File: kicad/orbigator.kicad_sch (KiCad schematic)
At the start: 0 parts

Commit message: KiCad schematic WiP
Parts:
- added BT1: CR2032, symbol Device:Battery_Cell
- added DISP1: OLED_Encoder, symbol orbigator:OLED_Encoder
- added M1: DYNAMIXEL_1, symbol Connector_Generic:Conn_01x03
- added M2: DYNAMIXEL_2, symbol Connector_Generic:Conn_01x03
- added R1, R2, R3: 10k, symbol PCM_Elektuur:R
- added RTC1: DS3232, symbol orbigator:Adafruit_DS3231_Breakout
- added U1: Pico_2, Module_RaspberryPi_Pico:RaspberryPi_Pico_Original_SMD_HandSolder, symbol MCU_Module_RaspberryPi_Pico:RaspberryPi_Pico_DebugPins
- added U2: 74LS126, symbol 74xx:74LS126
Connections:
- new net 3V3: DISP1.9 (VCC), R2.1 (+), R3.1 (+), RTC1.1 (Vin), U1.36 (3V3), U2.14 (VCC)
- new net 3V_BAT: BT1.1 (+), RTC1.5 (BAT)
- new net 5V0: M1.2 (Pin_2), M2.2 (Pin_2), R1.1 (+), U1.40 (VBUS)
- new net 5V_SYS: U1.39 (VSYS)
- new net BAK_BTN: DISP1.7 (BAK_BTN), U1.12 (GPIO9)
- new net CNF_BTN: DISP1.1 (CNF_BTN), U1.14 (GPIO10)
- new net DIR: U1.4 (GPIO2), U2.1
- new net ENC_A: DISP1.5 (ENC_A), U1.9 (GPIO6)
- new net ENC_B: DISP1.6 (ENC_B), U1.10 (GPIO7)
- new net ENC_SW: DISP1.4 (ENC_SW), U1.11 (GPIO8)
- new net GND: BT1.2 (-), DISP1.8 (GND), M1.1 (Pin_1), M2.1 (Pin_1), RTC1.2 (GND), U1.13 (GND), U1.18 (GND), U1.23 (GND), U1.28 (GND), U1.3 (GND), U1.38 (GND), U1.8 (GND), U1.D2 (GND), U2.10, U2.12, U2.13, U2.4, U2.5, U2.7 (GND), U2.9
- new net MOT_DAT: M1.3 (Pin_3), M2.3 (Pin_3), R1.2 (-), U1.2 (GPIO1), U2.3
- new net SCL: DISP1.3 (SCL), R2.2 (-), RTC1.3 (SCL), U1.7 (GPIO5)
- new net SDA: DISP1.2 (SDA), R3.2 (-), RTC1.4 (SDA), U1.6 (GPIO4)
- new net UART_TX: U1.1 (GPIO0), U2.2
- no-connect marks 0 -> 3
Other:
- company: WyoLum -> (none)
- title: Orbigator Controller -> (none)

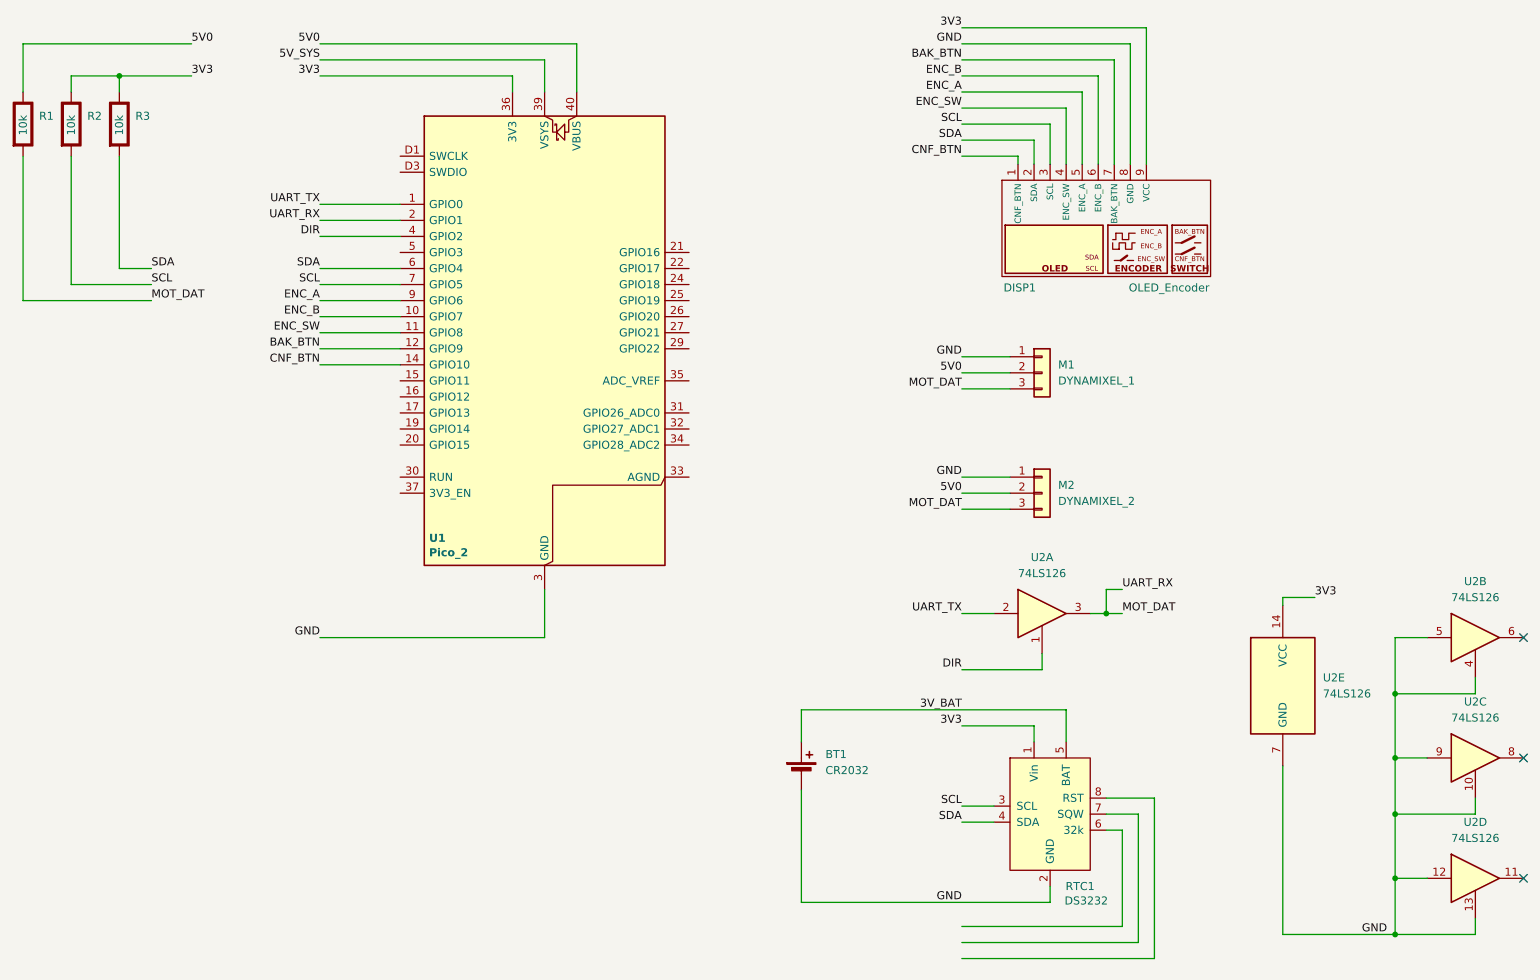
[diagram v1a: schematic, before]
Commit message: schematic done
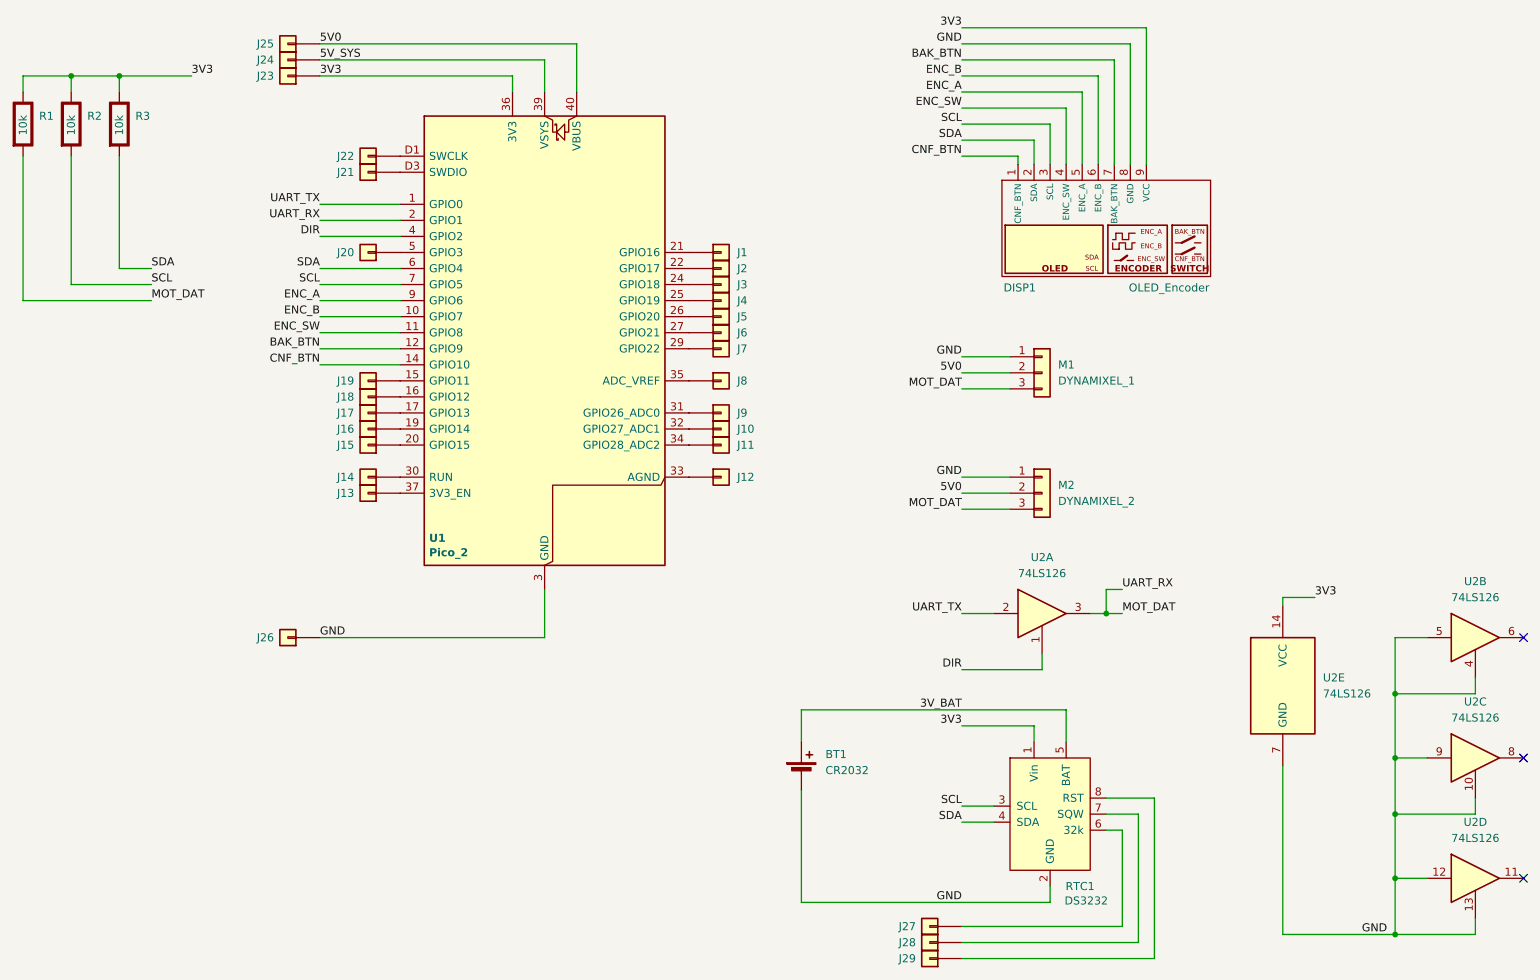
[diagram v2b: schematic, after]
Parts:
- added J1: Conn_01x01, symbol orbigator:Conn_01x01
- added J10: Conn_01x01, symbol orbigator:Conn_01x01_16
- added J11: Conn_01x01, symbol orbigator:Conn_01x01_15
- added J12: Conn_01x01, symbol orbigator:Conn_01x01_14
- added J13: Conn_01x01, symbol orbigator:Conn_01x01_13
- added J14: Conn_01x01, symbol orbigator:Conn_01x01_12
- added J15: Conn_01x01, symbol orbigator:Conn_01x01_11
- added J16: Conn_01x01, symbol orbigator:Conn_01x01_10
- added J17: Conn_01x01, symbol orbigator:Conn_01x01_9
- added J18: Conn_01x01, symbol orbigator:Conn_01x01_8
- added J19: Conn_01x01, symbol orbigator:Conn_01x01_7
- added J2: Conn_01x01, symbol orbigator:Conn_01x01_24
- added J20: Conn_01x01, symbol orbigator:Conn_01x01_6
- added J21: Conn_01x01, symbol orbigator:Conn_01x01_5
- added J22: Conn_01x01, symbol orbigator:Conn_01x01_4
- added J23: Conn_01x01, symbol orbigator:Conn_01x01_3
- added J24: Conn_01x01, symbol orbigator:Conn_01x01_2
- added J25, J26, J27, J28, J29: Conn_01x01, symbol orbigator:Conn_01x01_1
- added J3: Conn_01x01, symbol orbigator:Conn_01x01_23
- added J4: Conn_01x01, symbol orbigator:Conn_01x01_22
- added J5: Conn_01x01, symbol orbigator:Conn_01x01_21
- added J6: Conn_01x01, symbol orbigator:Conn_01x01_20
- added J7: Conn_01x01, symbol orbigator:Conn_01x01_19
- added J8: Conn_01x01, symbol orbigator:Conn_01x01_18
- added J9: Conn_01x01, symbol orbigator:Conn_01x01_17
- BT1: symbol Device:Battery_Cell -> orbigator:Battery_Cell
- M1, M2: symbol Connector_Generic:Conn_01x03 -> orbigator:Conn_01x03
- R1, R2, R3: symbol PCM_Elektuur:R -> orbigator:R
- U1: symbol MCU_Module_RaspberryPi_Pico:RaspberryPi_Pico_DebugPins -> orbigator:RaspberryPi_Pico_DebugPins
- U2: symbol 74xx:74LS126 -> orbigator:74LS126
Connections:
- net 3V3: now also R1.1 (+), J23.1 (Pin_1)
- net 5V0: now also J25.1 (Pin_1); no longer R1.1 (+)
- net 5V_SYS: now also J24.1 (Pin_1)
- net GND: now also J26.1 (Pin_1)
- net at U1.15 (GPIO11): now also J19.1 (Pin_1)
- net at U1.16 (GPIO12): now also J18.1 (Pin_1)
- net at U1.17 (GPIO13): now also J17.1 (Pin_1)
- net at U1.19 (GPIO14): now also J16.1 (Pin_1)
- net at U1.20 (GPIO15): now also J15.1 (Pin_1)
- net at U1.21 (GPIO16): now also J1.1 (Pin_1)
- net at U1.22 (GPIO17): now also J2.1 (Pin_1)
- net at U1.24 (GPIO18): now also J3.1 (Pin_1)
- net at U1.25 (GPIO19): now also J4.1 (Pin_1)
- net at U1.26 (GPIO20): now also J5.1 (Pin_1)
- net at U1.27 (GPIO21): now also J6.1 (Pin_1)
- net at U1.29 (GPIO22): now also J7.1 (Pin_1)
- net at U1.30 (RUN): now also J14.1 (Pin_1)
- net at U1.31 (GPIO26_ADC0): now also J9.1 (Pin_1)
- net at U1.32 (GPIO27_ADC1): now also J10.1 (Pin_1)
- net at U1.33 (AGND): now also J12.1 (Pin_1)
- net at U1.34 (GPIO28_ADC2): now also J11.1 (Pin_1)
- net at U1.35 (ADC_VREF): now also J8.1 (Pin_1)
- net at U1.37 (3V3_EN): now also J13.1 (Pin_1)
- net at U1.5 (GPIO3): now also J20.1 (Pin_1)
- net at U1.D1 (SWCLK): now also J22.1 (Pin_1)
- net at U1.D3 (SWDIO): now also J21.1 (Pin_1)
- net at RTC1.6 (32k): now also J27.1 (Pin_1)
- net at RTC1.7 (SQW): now also J28.1 (Pin_1)
- net at RTC1.8 (RST): now also J29.1 (Pin_1)
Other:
- company: (none) -> Wyolum
- title: (none) -> Orbigator PCB
